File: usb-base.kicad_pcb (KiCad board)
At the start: 4 copper layers, 100 x 100 mm, 19 parts, among them J1 USB3_B, U1 CYUSB3082-FCAXI, U2 TPS25221, U3 TPS62161DSG, U4 LFE5U-25F-6BG256C, U5 TPS62160DSG, U6 TPS62162DSG, Y1 24MHz, Y2 25MHz

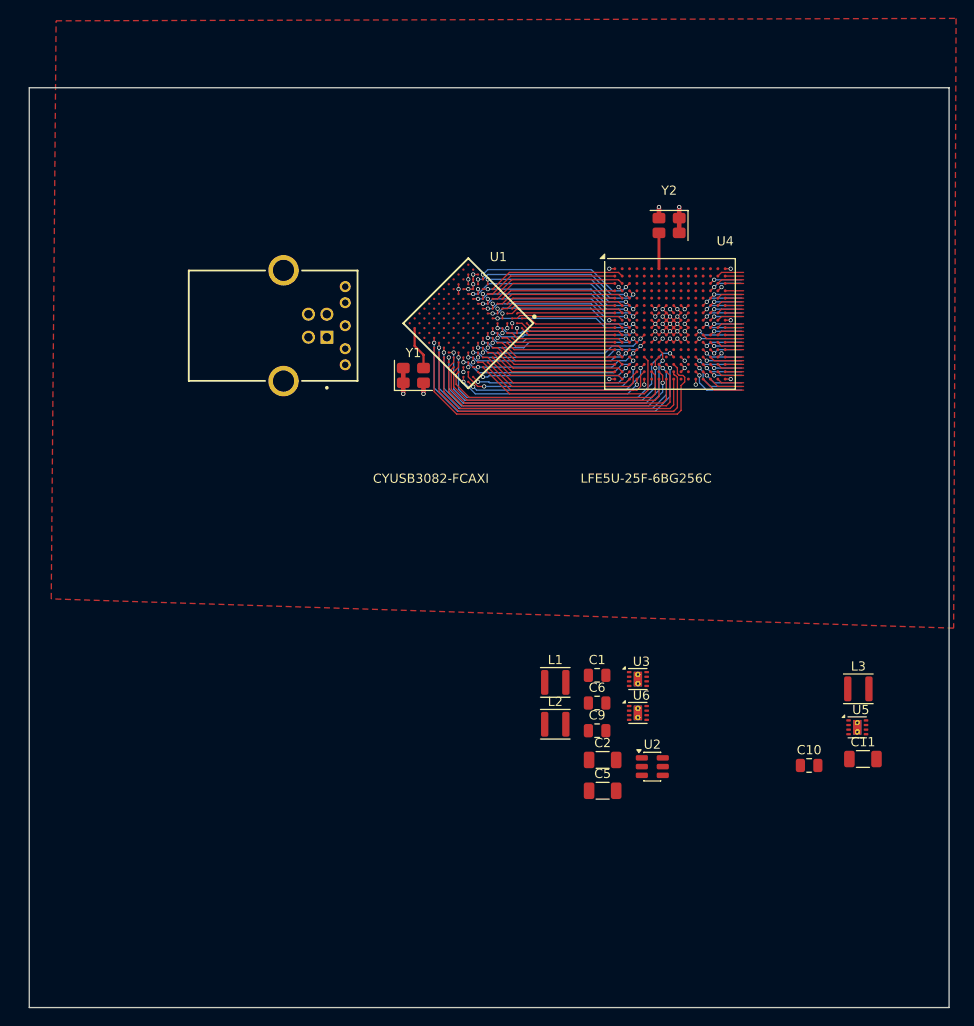
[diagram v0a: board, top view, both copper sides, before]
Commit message: lots of work on layout
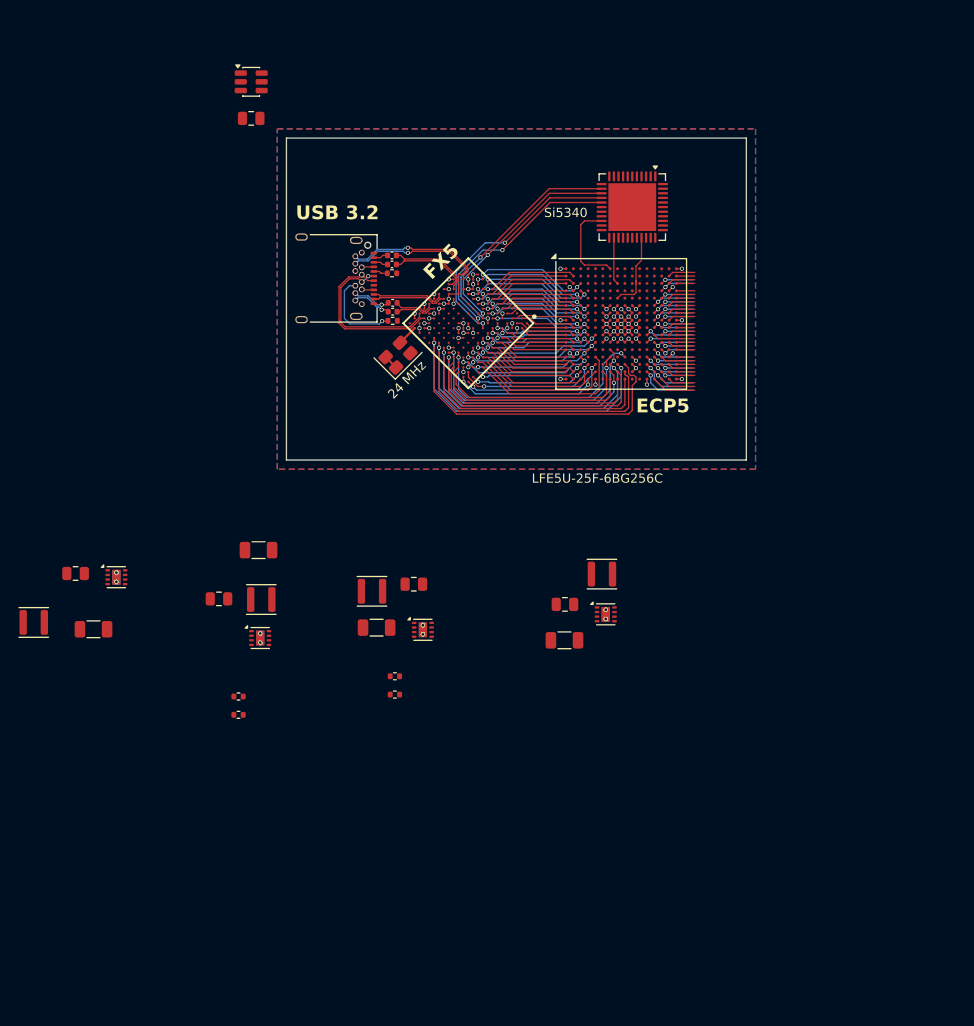
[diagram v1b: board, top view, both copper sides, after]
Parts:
- removed J1: USB3_B, Infineon:SAMTEC_USB3-B-S-F-TH
- removed Y2: 25MHz, Crystal:Crystal_SMD_SeikoEpson_TSX3225-4Pin_3.2x2.5mm
- added C12: 100n, Capacitor_SMD:C_0402_1005Metric, F.Cu at (114.5, 56.9)
- added C13: 100n, Capacitor_SMD:C_0402_1005Metric, F.Cu at (114.5, 57.9)
- added C14: 10u, Capacitor_SMD:C_0805_2012Metric, F.Cu at (116.8, 87.5)
- added C15: 22u, Capacitor_SMD:C_1206_3216Metric, F.Cu at (112.8, 92.2)
- added C7: 100n, Capacitor_SMD:C_0402_1005Metric, F.Cu at (114.5, 52.7)
- added C8: 100n, Capacitor_SMD:C_0402_1005Metric, F.Cu at (114.5, 51.8)
- added J2: USB_C_Receptacle, Connector_USB:USB_C_Receptacle_Amphenol_12401548E4-2A, F.Cu at (107.5, 54.2)
- added L4: 2.2u, Inductor_SMD:L_Sunlord_SWPA3015S, F.Cu at (112.3, 88.3)
- added R4: 20k, Resistor_SMD:R_0402_1005Metric, F.Cu at (97.8, 99.7)
- added R5: 7.5k, Resistor_SMD:R_0402_1005Metric, F.Cu at (97.8, 101.7)
- added R6: R, Resistor_SMD:R_0402_1005Metric, F.Cu at (114.8, 97.5)
- added R7: R, Resistor_SMD:R_0402_1005Metric, F.Cu at (114.8, 99.5)
- added R8: R, Resistor_SMD:R_0402_1005Metric, F.Cu at (114.5, 58.9)
- added R9: R, Resistor_SMD:R_0402_1005Metric, F.Cu at (114.5, 53.7)
- added U7: Si5340, Package_DFN_QFN:QFN-44-1EP_7x7mm_P0.5mm_EP5.2x5.2mm, F.Cu at (140.6, 46.5)
- added U8: TPS62160DSG, Package_SON:WSON-8-1EP_2x2mm_P0.5mm_EP0.9x1.6mm_ThermalVias, F.Cu at (117.8, 92.5)
- U1: footprint Infineon:BGA169N075P13X13_10X10X120 -> library:BGA169N075P13X13_10X10X120
- moved U2 86.3 mm to (99.2, 32.9)
- moved C9 76.5 mm to (99.2, 36.9)
- moved C11 69.5 mm to (100.0, 83.8)
- moved C10 66.7 mm to (95.7, 89.1)
- moved L3 65.6 mm to (100.3, 89.2)
- moved U5 65.6 mm to (100.2, 93.3)
- moved C1 57.8 mm to (80.1, 86.3)
- moved U3 57.8 mm to (84.5, 86.7)
- moved L2 57.8 mm to (75.5, 91.7)
- moved C2 57.1 mm to (82.0, 92.4)
- moved C5 16.9 mm to (133.2, 93.6)
- moved L1 12.8 mm to (137.3, 86.4)
- moved C6 11.3 mm to (133.3, 89.7)
- moved U6 11.3 mm to (137.7, 90.8)
- moved U4 5.30 mm to (139.4, 59.2)
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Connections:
- net +1V8 renamed +1.8V
- net +2V5 renamed +2.5V
- net 24MHz renamed 24MHZ
- U1 pad A3: +3V3 -> +3.3V
- U1 pad C11: +3V3 -> +3.3V
- U1 pad C3: +3V3 -> +3.3V
- U1 pad C5: +3V3 -> +3.3V
- U1 pad C7: +3V3 -> +3.3V
- U1 pad C9: +3V3 -> +3.3V
- U1 pad E3: +3V3 -> +3.3V
- U1 pad E5: unconnected-(U1C-P7_2_SPIDAT2-PadE5) -> CLK_SPI_MOSI
- U1 pad E6: unconnected-(U1C-P7_3_SPIDAT3-PadE6) -> CLK_SPI_MISO
- U1 pad F5: unconnected-(U1C-P7_0_SPIDAT0-PadF5) -> CLK_SPI_CLK
- U1 pad F6: unconnected-(U1C-P7_1_SPIDAT1-PadF6) -> CLK_SPI_CS
- U1 pad F7: +3V3 -> +3.3V
- U1 pad G3: +3V3 -> +3.3V
- U1 pad J3: +3V3 -> +3.3V
- U1 pad L10: +3V3 -> +3.3V
- U1 pad L13: +3V3 -> +3.3V
- U1 pad M12: +3V3 -> +3.3V
- U1 pad M3: USBSS_RX+ -> USBSS_RX1+
- U1 pad M5: USBSS_TX+ -> USBSS_TX1+
- U1 pad M7: unconnected-(U1B-USB3TX2_P-PadM7) -> USBSS_RX2+
- U1 pad M9: unconnected-(U1B-USB3RX2_P-PadM9) -> USBSS_TX2+
- U1 pad N3: USBSS_RX- -> USBSS_RX1-
- U1 pad N5: USBSS_TX- -> USBSS_TX1-
- U1 pad N7: unconnected-(U1B-USB3TX2_N-PadN7) -> USBSS_RX2-
- U1 pad N9: unconnected-(U1B-USB3RX2_N-PadN9) -> USBSS_TX2-
- U4 pad A7: 25MHz -> 100MHZ
- U4 pad C8: unconnected-(U4C-PT44A/+/PCLKT1_0-PadC8) -> CLK2
- U4 pad E8: unconnected-(U4C-PT42A/+/PCLKT1_1-PadE8) -> CLK1
- U4 pad F10: +3V3 -> +3.3V
- U4 pad F11: +3V3 -> +3.3V
- U4 pad F6: +3V3 -> +3.3V
- U4 pad F7: +3V3 -> +3.3V
- U4 pad H11: +3V3 -> +3.3V
- U4 pad H6: +3V3 -> +3.3V
- U4 pad H7: +3V3 -> +3.3V
- U4 pad J11: +3V3 -> +3.3V
- U4 pad J6: +3V3 -> +3.3V
- U4 pad J7: +3V3 -> +3.3V
- U4 pad K11: +3V3 -> +3.3V
- U4 pad L11: +3V3 -> +3.3V
- U4 pad L6: +3V3 -> +3.3V
- U4 pad N10: +3V3 -> +3.3V
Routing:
- net CLK_SPI_MISO: track 0.00 -> 26.8 mm, vias 0 -> 2
- net CLK_SPI_MOSI: track 0.00 -> 25.8 mm, vias 0 -> 2
- net CLK_SPI_CS: track 0.00 -> 25.0 mm, vias 0 -> 2
- net CLK_SPI_CLK: track 0.00 -> 24.0 mm, vias 0 -> 2
- net USBHS_D-: track 0.00 -> 18.6 mm
- net USBHS_D+: track 0.00 -> 17.8 mm, vias 0 -> 1
- net USBSS_RX1+: track 0.00 -> 15.2 mm, vias 0 -> 1
- net USBSS_RX1-: track 0.00 -> 14.7 mm, vias 0 -> 1
- net +3V3: track 13.8 -> 0.00 mm, vias 17 -> 0
- net +3.3V: track 5.60 -> 17.5 mm, vias 2 -> 20
- net P0D14: track 10.7 -> 0.10 mm
- net 100MHZ: track 0.00 -> 9.96 mm
- net Net-(J2-CC2): track 0.00 -> 9.54 mm, vias 0 -> 1
- net USBSS_TX1+: track 0.00 -> 9.15 mm
- net CLK1: track 0.00 -> 8.80 mm
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- added copper zone on B.Cu, net GND
- added copper zone on In2.Cu, net GND
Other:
- board size 100 x 100 mm -> 50 x 35 mm
- board text added: "24 MHz"
- board text added: "ECP5"
- board text added: "FX5"
- board text added: "Si5340"
- board text added: "USB 3.2"
